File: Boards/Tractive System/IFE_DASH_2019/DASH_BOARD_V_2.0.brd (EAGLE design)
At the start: 160 x 100 mm, 77 parts, among them IC1 STM32F10XCXT6

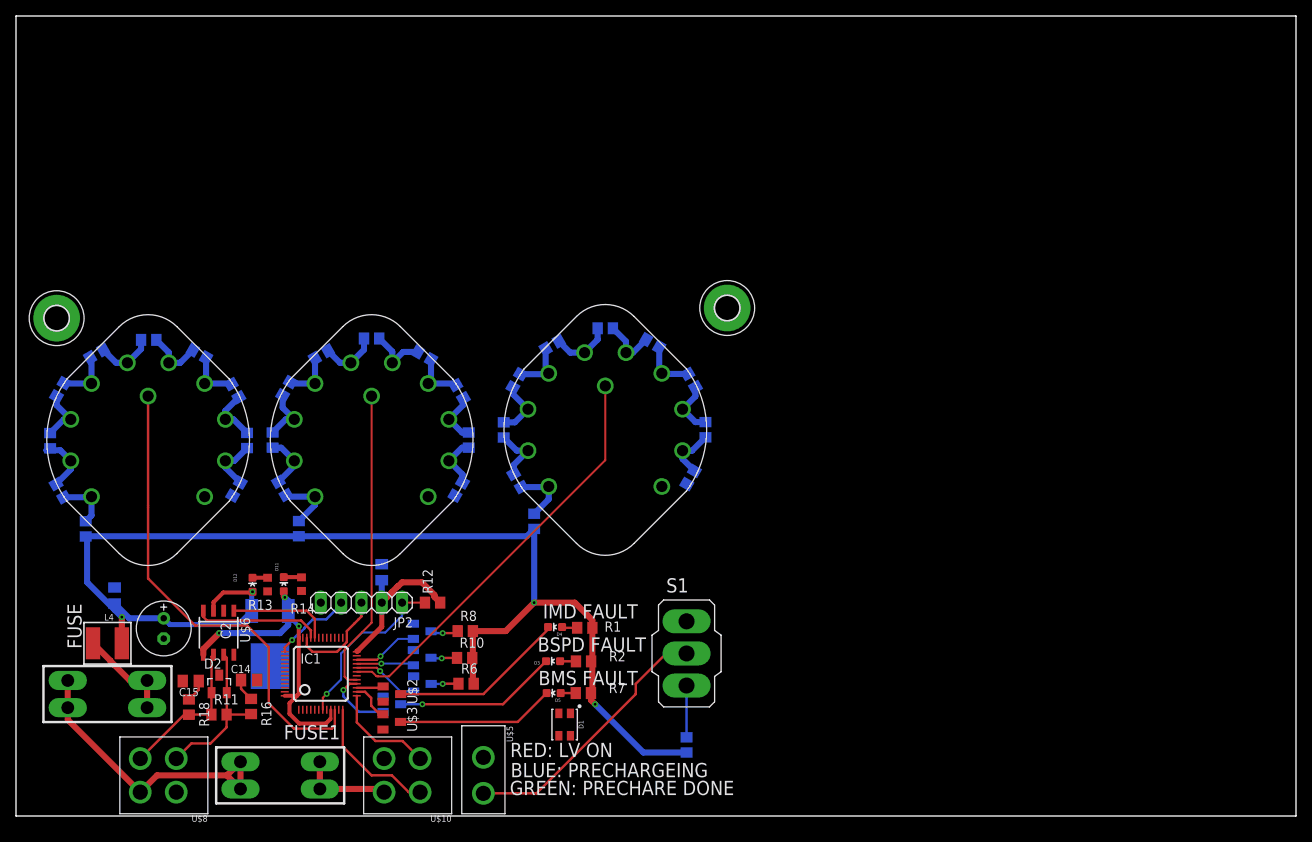
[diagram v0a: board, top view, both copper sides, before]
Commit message: v2 done
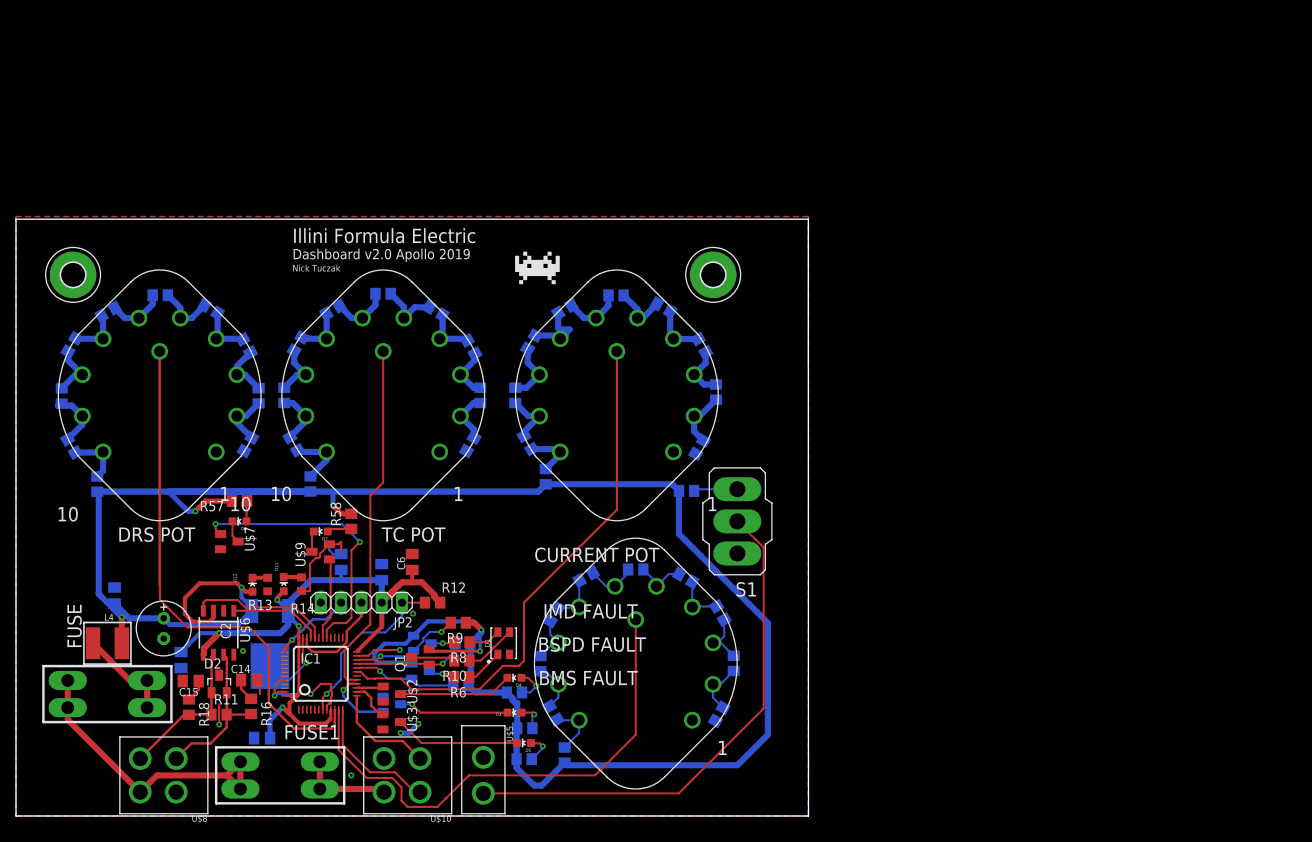
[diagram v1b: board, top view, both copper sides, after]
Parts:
- removed U$11, U$12: DMN2300U, Display_Custom:SOT23
- added C1, C3, C4, C6: 0.1u, rcl:C0805K
- added CUSTOM_POT: SWITCH_ROTARY_1X10KIT, Testing:ROTARY_SWITCH_1X10_KIT
- added D6: DRS_BLUE, SparkFun-LED:LED-0603
- added D7: TC_BLUE, SparkFun-LED:LED-0603
- added Q1, Q2, Q6: DMP3099L-7, TRANS:SOT23
- added R4, R47, R48, R49, R5, R50, R51, R52, R53, R54, R55, R9: 10k, resistor:R0805
- added R56: 1k, resistor:R0805
- added R57, R58: 330, resistor:R0805
- added U$7: DMN2300U, Display_Custom:SOT23
- R1, R2, R7: value 10k -> 330
- R10: value 1k -> 85
- R13, R14: value (none) -> 330
- R6: value 1k -> 140
- R8: value 1k -> 90
- moved R3 31.8 mm to (83.8, 40.6), turned to 0 degrees
- moved U$9 20.8 mm to (38.1, 33.0), flipped to the top
- moved S1 17.7 mm to (90.2, 36.8), turned to 180 degrees
- moved D1 12.7 mm to (61.0, 21.6), turned to 90 degrees
- moved R1 11.9 mm to (62.3, 15.4), flipped to the bottom
- moved R2 11.1 mm to (63.6, 11.0), flipped to the bottom
- moved R7 11.1 mm to (63.5, 7.11), flipped to the bottom
- moved D4 8.13 mm to (62.3, 17.3)
- moved D3 8.02 mm to (62.3, 12.9)
- moved D5 7.27 mm to (63.5, 9.12)
- moved H6 5.79 mm to (7.14, 67.6), turned to 180 degrees
- moved R30 5.77 mm to (45.9, 65.3)
- moved DRS_POT 5.77 mm to (18.0, 52.6)
- moved R26 5.77 mm to (34.7, 46.5)
- moved R27 5.77 mm to (33.5, 52.6)
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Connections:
- removed net CAN_RX/STM_TX: IC1.33, U$6.4
- removed net CAN_TX/STM_RX: IC1.32, U$6.1
- removed net DASH_POWER_ON: IC1.20, U$9.1
- removed net DASH_PRE_DONE: IC1.22, U$12.1
- removed net DASH_PRE_STARTED: IC1.21, U$11.1
- new net CAN_RX: IC1.32, U$6.4
- new net CAN_TX: IC1.33, U$6.1
- new net CUSTOM_VALUE: CUSTOM_POT.COMMON, IC1.11
- new net DRS_: D6.A, R57.1
- new net DRS_LED: IC1.29, U$7.1
- new net N$1: Q6.3, R6.2
- new net N$24: Q1.3, R10.2
- new net N$27: Q2.3, R8.2
- new net N$34: CUSTOM_POT.2, R47.2, R48.1
- new net N$35: CUSTOM_POT.3, R48.2, R49.2
- new net N$45: CUSTOM_POT.4, R49.1, R50.2
- new net N$46: CUSTOM_POT.5, R50.1, R51.2
- new net N$47: CUSTOM_POT.6, R51.1, R52.2
- new net N$48: CUSTOM_POT.7, R52.1, R53.2
- new net N$49: CUSTOM_POT.8, R53.1, R54.2
- new net N$50: CUSTOM_POT.9, R54.1, R55.2
- new net N$51: CUSTOM_POT.1, R47.1, R56.1
- new net N$52: D6.C, U$7.3
- new net N$53: D7.C, U$9.3
- new net RGB_BLUE: IC1.21, Q1.1, R5.2
- new net RGB_GREEN: IC1.22, Q2.1, R9.2
- new net RGB_RED: IC1.20, Q6.1, R4.2
- new net TC_: D7.A, R58.1
- new net TC_LED: IC1.30, U$9.1
- net +3V3: now also C1.1, C3.1, C4.1, C6.1
- net +5V: now also Q1.2, Q2.2, Q6.2, R4.1, R5.1, R56.2, R57.2, R58.2, R9.1; no longer R10.2, R6.2, R8.2
- net GND: now also C1.2, C3.2, C4.2, C6.2, CUSTOM_POT.10, R55.1, U$7.2; no longer U$11.2, U$12.2
- net N$15: no longer U$11.3
- net N$16: no longer U$9.3
- net N$5: no longer U$12.3
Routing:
- net +5V: track 158.1 -> 291.2 mm, vias 4 -> 6
- net CUSTOM_VALUE: track 0.00 -> 64.2 mm
- net GND: track 0.00 -> 51.6 mm, vias 0 -> 10
- net DRS_LED: track 0.00 -> 35.1 mm, vias 0 -> 2
- net ENABLE: track 33.4 -> 64.2 mm
- net +3V3: track 59.3 -> 88.1 mm, vias 3 -> 4
- net CAN_RX: track 0.00 -> 17.8 mm
- net CAN_RX/STM_TX: track 15.9 -> 0.00 mm
- net CURRENT_VALUE: track 51.8 -> 66.8 mm
- net RGB_BLUE: track 0.00 -> 14.0 mm, vias 0 -> 1
- net RGB_GREEN: track 0.00 -> 13.9 mm, vias 0 -> 2
- net RGB_RED: track 0.00 -> 13.0 mm, vias 0 -> 1
- net CAN_TX/STM_RX: track 12.9 -> 0.00 mm
- net CAN_TX: track 0.00 -> 11.6 mm
- net DASH_PRE_DONE: track 10.6 -> 0.00 mm, vias 1 -> 0
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- added copper zone on layer 1, net GND
- added copper zone on layer 16, net GND
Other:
- board size 160 x 100 mm -> 99.1 x 74.6 mm
- board text added: "1"
- board text added: "10"
- board text added: "CURRENT POT"
- board text added: "DRS POT"
- board text added: "Dashboard v2.0 Apollo 2019"
- board text added: "Illini Formula Electric"
- board text added: "Nick Tuczak"
- board text added: "TC POT"
- board text removed: "BLUE: PRECHARGEING"
- board text removed: "GREEN: PRECHARE DONE"
- board text removed: "RED: LV ON"
